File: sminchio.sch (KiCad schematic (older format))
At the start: 9 parts, among them J1 Screw_Terminal_01x06, Q1 SQ4435EY, Q2 SQ4435EY, U1 LTC4412xS6, U2 LTC4412xS6

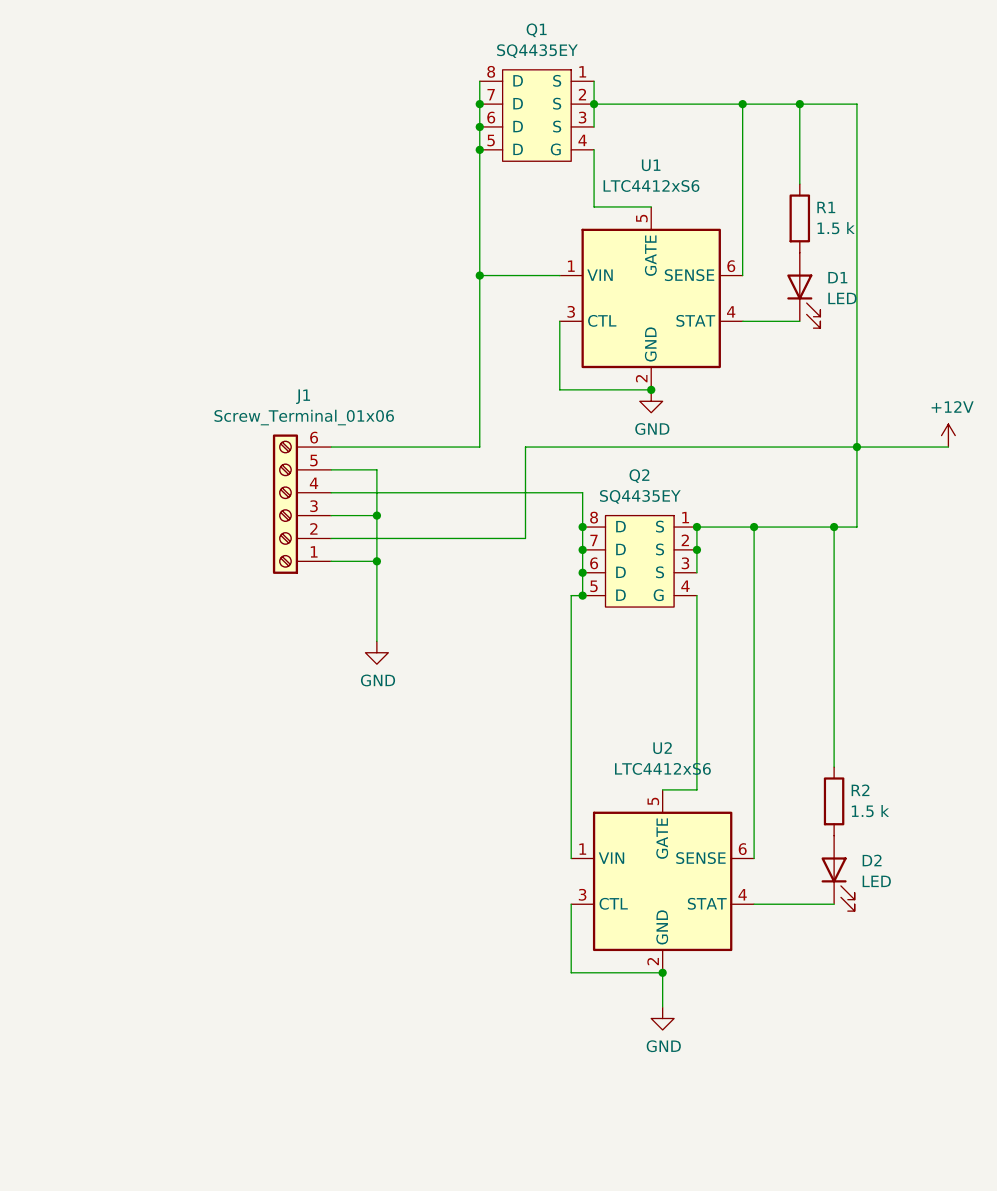
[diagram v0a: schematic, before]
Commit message: Almost complete version
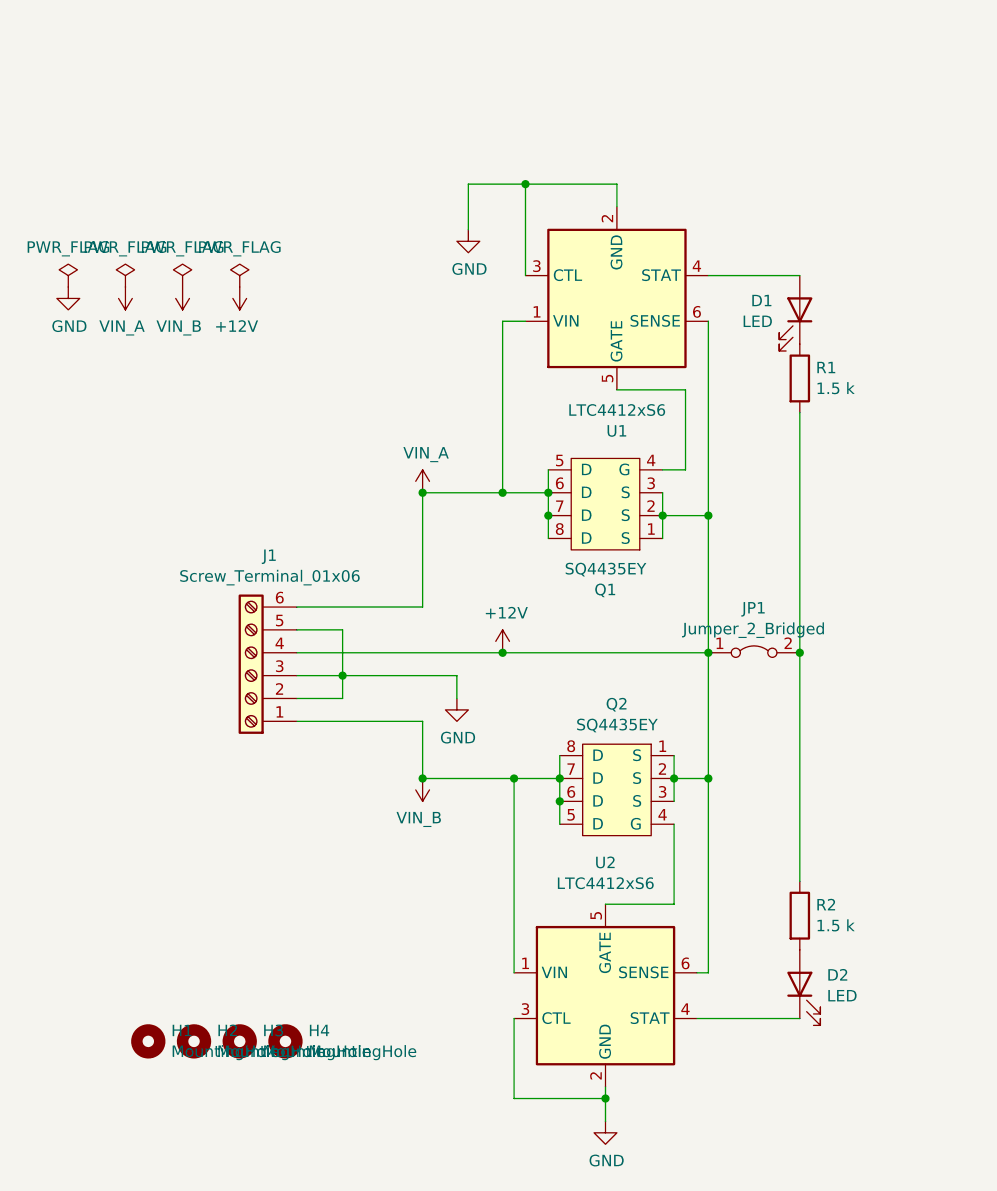
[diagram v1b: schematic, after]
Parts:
- added H1, H2, H3, H4: MountingHole, Mounting_Holes:MountingHole_2.2mm_M2, symbol Mechanical:MountingHole
- added JP1: Jumper_2_Bridged, Pin_Headers:Pin_Header_Straight_1x02_Pitch2.54mm, symbol Jumper:Jumper_2_Bridged
- U1, U2: footprint TO_SOT_Packages_SMD:TSOT-23-6 -> Package_TO_SOT_SMD:TSOT-23-6
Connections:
- net +12V: now also J1.4 (Pin_4), JP1.1 (A); no longer J1.2 (Pin_2), R1.1, R2.1
- net GND: now also J1.2 (Pin_2); no longer J1.1 (Pin_1)
- net VIN_B: now reaches Q2.5 (D), Q2.6 (D), Q2.7 (D), Q2.8 (D), U2.1 (VIN)
- net VIN_B: now also J1.1 (Pin_1); no longer J1.4 (Pin_4)
- net VIN_A: now reaches J1.6 (Pin_6), Q1.5 (D), Q1.6 (D), Q1.7 (D), Q1.8 (D), U1.1 (VIN)
- net at U1.4 (STAT): now also D1.2 (A); no longer D1.1 (K)
- net at R1.2: now also R2.1, JP1.2 (B); no longer D1.2 (A)
- new net: D1.1 (K), R1.1
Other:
- moved on the sheet: D1, D2, J1, Q1, Q2, R1, R2, U1, U2
